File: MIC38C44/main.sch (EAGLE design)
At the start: 59 parts, among them Q1 800-1000V

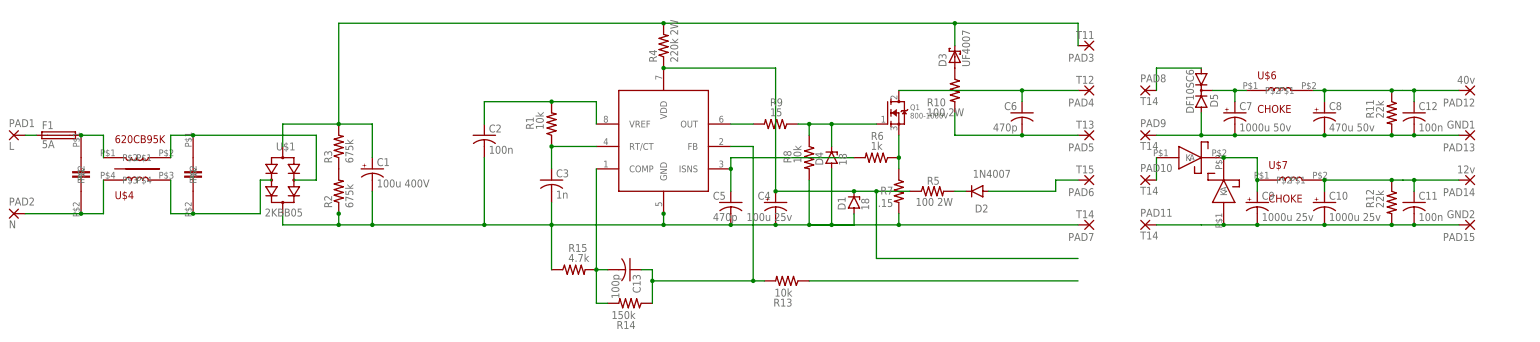
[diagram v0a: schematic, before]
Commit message: -a
a
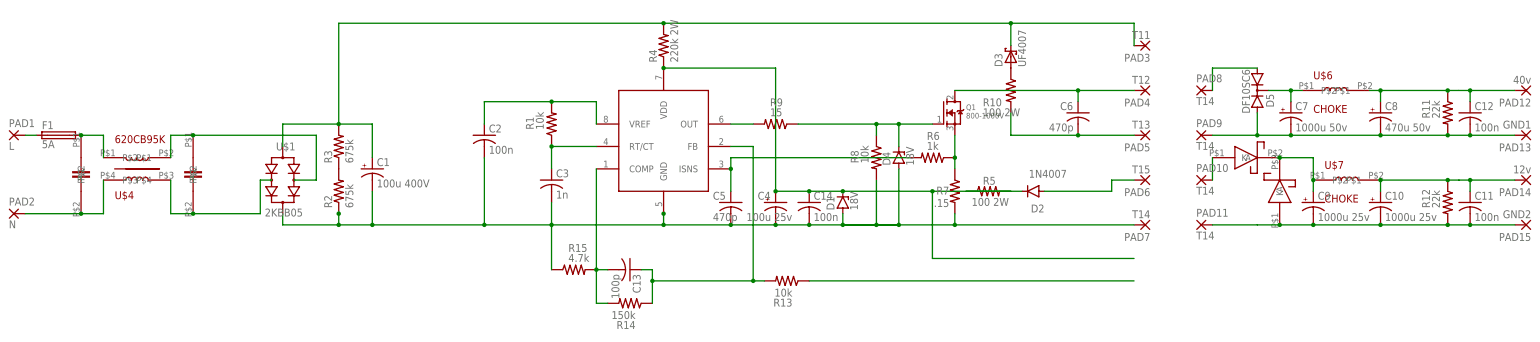
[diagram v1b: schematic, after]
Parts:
- added C14: 100n, rcl:C-US050-035X075
- D1, D4: value 18 -> 18V
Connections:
- net GND: now also C14.2
- net N$11: now also R5.1; no longer R5.2
- net VDD: now also C14.1, R5.2; no longer R5.1
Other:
- moved on the sheet: C10, C11, C12, C6, C7, C8, C9, D1, D2, D3, D4, D5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
